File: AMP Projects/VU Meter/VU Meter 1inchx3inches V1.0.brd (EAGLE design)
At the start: 25.4 x 76.2 mm, 23 parts, among them IC1 LM3914N

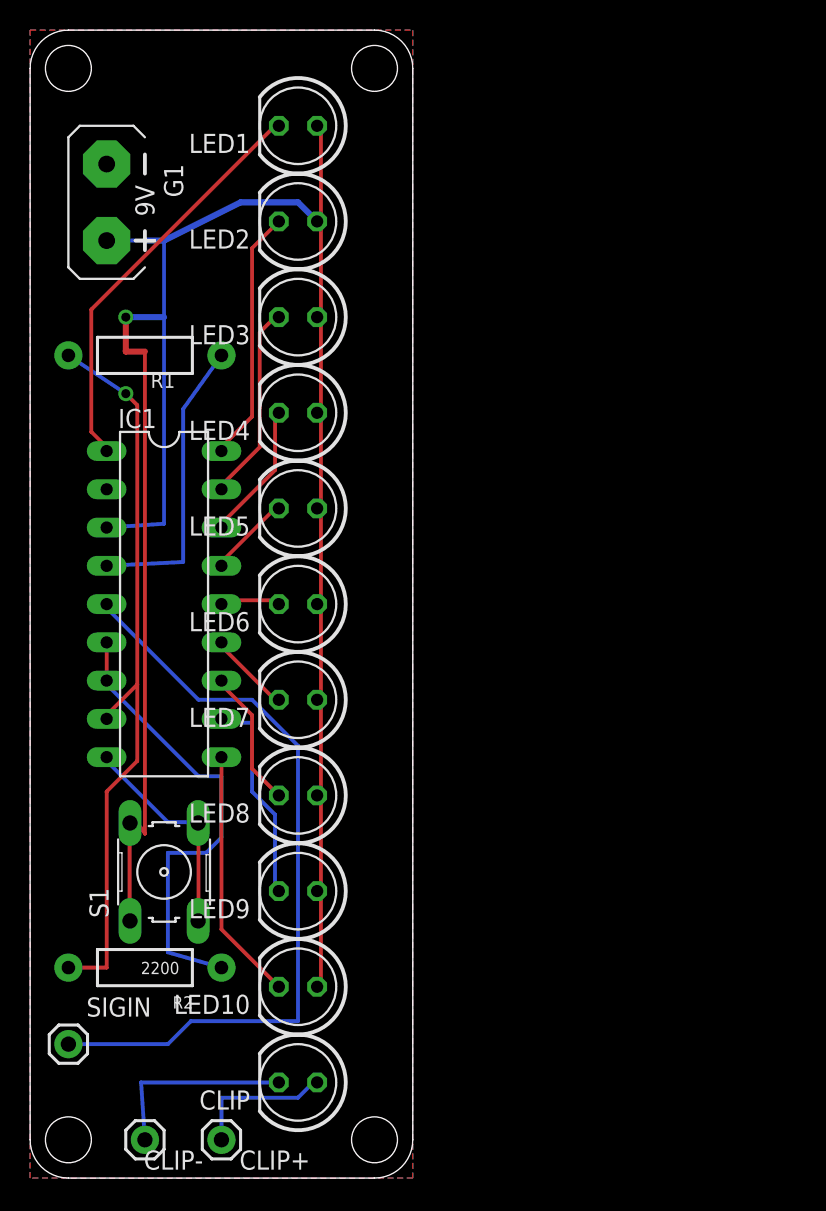
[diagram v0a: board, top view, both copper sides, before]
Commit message: Updates to most boards
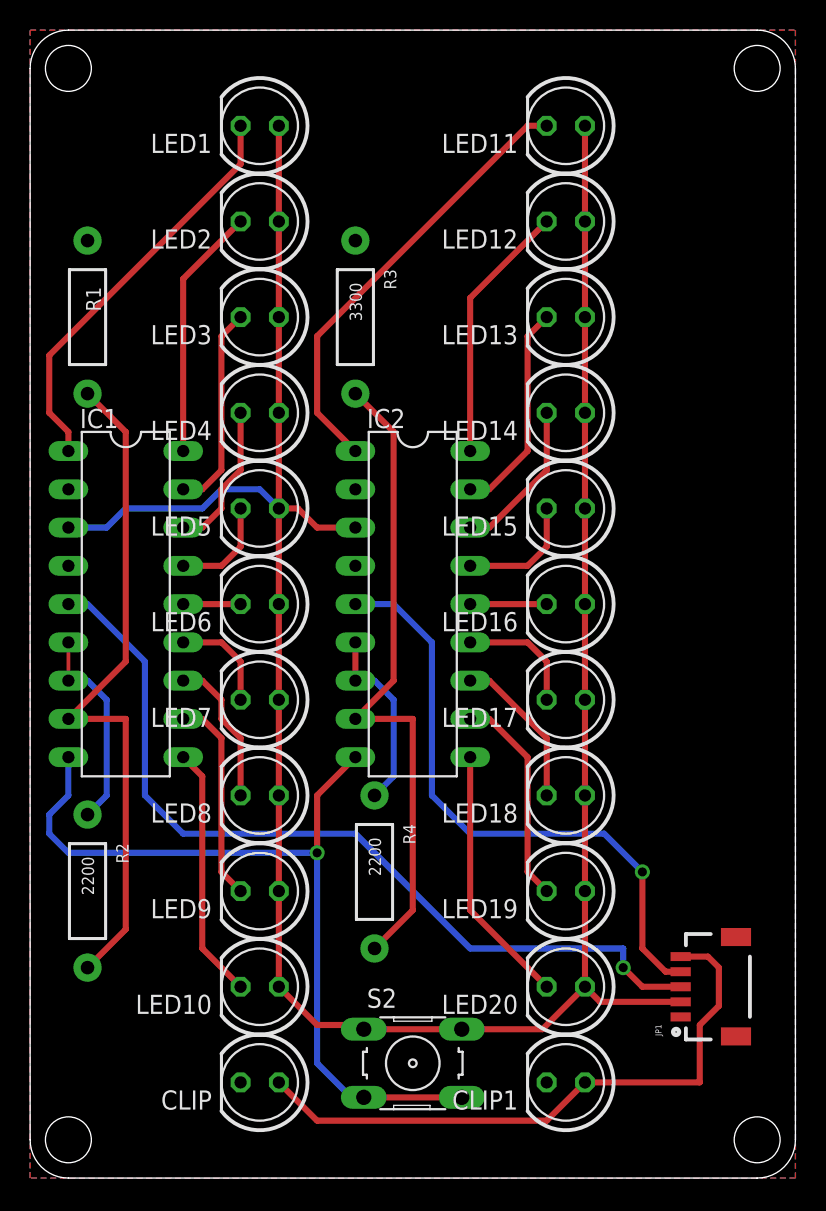
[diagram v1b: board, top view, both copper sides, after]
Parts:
- removed CLIP+, CLIP-, SIGIN: M01PTH, SparkFun-Connectors:1X01
- removed G1: AB9V, battery:AB9V
- removed S1: (no value), switch-omron:B3F-10XX
- added CLIP1, LED11, LED12, LED13, LED14, LED15, LED16, LED17, LED18, LED19, LED20: (no value), led:LED5MM
- added IC2: LM3914N, national-semiconductor:DIL18
- added JP1: (no value), SparkFun-Connectors:1X05-1MM-RA
- added R3: 3300, SparkFun-Resistors:AXIAL-0.4
- added R4: 2200, SparkFun-Resistors:AXIAL-0.4
- added S2: (no value), switch-omron:B3F-10XX
- moved U$1 25.4 mm to (48.3, 73.7)
- moved U$2 25.4 mm to (48.3, 2.54)
- moved R2 6.35 mm to (3.81, 19.1), turned to 270 degrees
- moved R1 4.58 mm to (3.81, 57.1), turned to 270 degrees
- moved CLIP 2.54 mm to (15.2, 6.35)
- moved IC1 2.54 mm to (6.35, 38.1)
- moved LED1 2.54 mm to (15.2, 69.8)
- moved LED10 2.54 mm to (15.2, 12.7)
- moved LED2 2.54 mm to (15.2, 63.5)
- moved LED3 2.54 mm to (15.2, 57.1)
- moved LED4 2.54 mm to (15.2, 50.8)
- moved LED5 2.54 mm to (15.2, 44.5)
- moved LED6 2.54 mm to (15.2, 38.1)
- moved LED7 2.54 mm to (15.2, 31.8)
- moved LED8 2.54 mm to (15.2, 25.4)
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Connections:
- removed net N$15: IC1.9, S1.3, S1.4
- new net CLIP+: CLIP.A, CLIP1.A, JP1.5
- new net L-SIG: IC1.5, JP1.3
- new net MODE: IC1.9, IC2.9, S2.3, S2.4
- new net N$14: IC2.6, IC2.7, R4.P$1
- new net N$19: IC2.16, LED14.K
- new net N$20: IC2.15, LED15.K
- new net N$21: IC2.14, LED16.K
- new net N$23: IC2.13, LED17.K
- new net N$24: IC2.12, LED18.K
- new net N$25: IC2.11, LED19.K
- new net N$26: IC2.10, LED20.K
- new net N$27: IC2.8, R3.P$2, R4.P$2
- new net R-SIG: IC2.5, JP1.4
- net GND: now also CLIP.K, CLIP1.K, IC2.2, IC2.4, JP1.1, R3.P$1; no longer G1.-
- net N$16: now also IC2.1, LED11.K; no longer IC1.5, SIGIN.1
- net N$17: now also IC2.18, LED12.K; no longer CLIP+.1, CLIP.A
- net N$18: now also IC2.17, LED13.K; no longer CLIP-.1, CLIP.K
- net V+: now also IC2.3, JP1.2, LED11.A, LED12.A, LED13.A, LED14.A, LED15.A, LED16.A, LED17.A, LED18.A, LED19.A, LED20.A, S2.1, S2.2; no longer G1.+, S1.1, S1.2
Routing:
- net L-SIG: track 0.00 -> 57.1 mm, vias 0 -> 1
- net MODE: track 0.00 -> 55.8 mm, vias 0 -> 1
- net N$27: track 0.00 -> 43.8 mm
- net CLIP+: track 0.00 -> 41.0 mm
- net R-SIG: track 0.00 -> 40.6 mm, vias 0 -> 1
- net V+: track 143.1 -> 164.9 mm, vias 1 -> 0
- net N$16: track 50.9 -> 29.7 mm
- net GND: track 19.6 -> 0.00 mm
- net N$2: track 31.3 -> 13.8 mm
- net N$26: track 0.00 -> 17.3 mm
- net N$15: track 14.5 -> 0.00 mm
- net N$25: track 0.00 -> 14.3 mm
- net N$14: track 0.00 -> 12.5 mm
- net N$24: track 0.00 -> 10.5 mm
- net N$19: track 0.00 -> 10.5 mm
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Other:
- board size 25.4 x 76.2 mm -> 50.8 x 76.2 mm
